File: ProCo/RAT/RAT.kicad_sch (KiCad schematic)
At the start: 40 parts, among them J1 I/O, J2 Power, J3 Power, Q1 2N5458, SW1 SW_SPDT, U1 LM308N

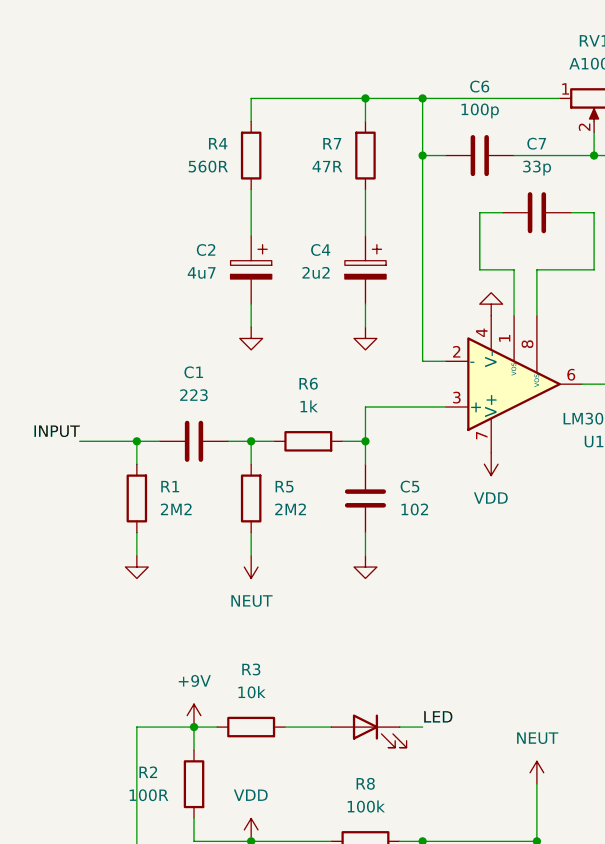
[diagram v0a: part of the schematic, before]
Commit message: refactor: 見直しに伴う形式的な更新
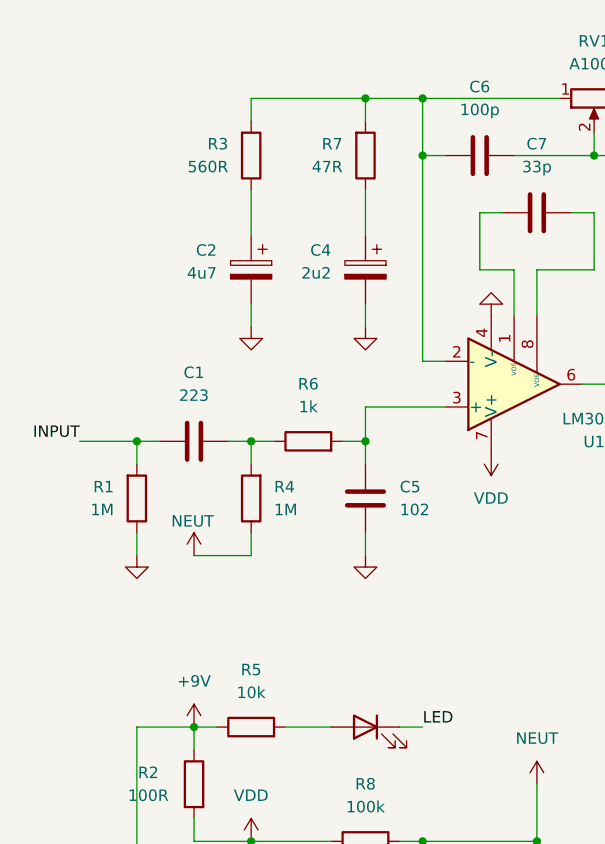
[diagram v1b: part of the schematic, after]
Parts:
- R1: value 2M2 -> 1M
- R4: renamed from R5; value 2M2 -> 1M
- renumbered R4 to R3, R3 to R5
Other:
- moved on the sheet: R1
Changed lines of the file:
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@@
 	(wire
 		(pts
+			(xy 38.1 82.55) (xy 44.45 82.55)
+		)
+		(stroke
+			(width 0)
+			(type default)
+		)
+	)
+	(wire
+		(pts
 			(xy 76.2 107.95) (xy 76.2 114.3)
 		)
@@
 	(wire
 		(pts
+			(xy 44.45 82.55) (xy 44.45 80.01)
+		)
+		(stroke
+			(width 0)
+			(type default)
+		)
+	)
+	(wire
+		(pts
 			(xy 158.75 50.8) (xy 158.75 31.75)
 		)
@@
 	(wire
 		(pts
-			(xy 44.45 80.01) (xy 44.45 82.55)
-		)
-		(stroke
-			(width 0)
-			(type default)
-		)
-	)
-	(wire
-		(pts
 			(xy 44.45 69.85) (xy 44.45 72.39)
 		)
@@
 		(dnp no)
 		(fields_autoplaced yes)
-		(property "Reference" "#PWR025"
+		(property "Reference" "#PWR027"
 			(at 177.8 88.9 0)
 			(hide yes)
@@
 			(project "RAT"
 				(path "/938e6a14-1226-49e6-a6eb-20951bcd3e89"
-					(reference "#PWR025")
+					(reference "#PWR027")
 					(unit 1)
 				)
@@
 		(dnp no)
 		(fields_autoplaced yes)
-		(property "Reference" "#PWR02"
+		(property "Reference" "#PWR03"
 			(at 38.1 105.41 0)
 			(hide yes)
@@
 			(project "RAT"
 				(path "/938e6a14-1226-49e6-a6eb-20951bcd3e89"
-					(reference "#PWR02")
+					(reference "#PWR03")
 					(unit 1)
 				)
@@
 	(symbol
 		(lib_id "Device:R")
-		(at 31.75 76.2 180)
+		(at 31.75 76.2 0)
+		(mirror x)
 		(unit 1)
 		(body_style 1)
@@
 		(in_pos_files yes)
 		(dnp no)
-		(fields_autoplaced yes)
 		(property "Reference" "R1"
-			(at 34.29 74.9299 0)
+			(at 29.21 74.9299 0)
 			(show_name no)
 			(do_not_autoplace no)
@@
 			)
 		)
-		(property "Value" "2M2"
-			(at 34.29 77.4699 0)
+		(property "Value" "1M"
+			(at 29.21 77.4699 0)
 			(show_name no)
 			(do_not_autoplace no)
@@
 		)
 		(property "Footprint" "Resistor_THT:R_Axial_DIN0207_L6.3mm_D2.5mm_P7.62mm_Horizontal"
-			(at 33.528 76.2 90)
+			(at 29.972 76.2 90)
 			(hide yes)
 			(show_name no)
@@
 		(dnp no)
 		(fields_autoplaced yes)
-		(property "Reference" "#PWR023"
+		(property "Reference" "#PWR025"
 			(at 171.45 40.64 0)
 			(hide yes)
@@
 			(project "RAT"
 				(path "/938e6a14-1226-49e6-a6eb-20951bcd3e89"
-					(reference "#PWR023")
+					(reference "#PWR025")
 					(unit 1)
 				)
@@
 		(dnp no)
 		(fields_autoplaced yes)
-		(property "Reference" "R5"
+		(property "Reference" "R4"
 			(at 46.99 74.9299 0)
 			(show_name no)
@@
 			)
 		)
-		(property "Value" "2M2"
+		(property "Value" "1M"
 			(at 46.99 77.4699 0)
 			(show_name no)
@@
 			(project "RAT"
 				(path "/938e6a14-1226-49e6-a6eb-20951bcd3e89"
-					(reference "R5")
+					(reference "R4")
 					(unit 1)
 				)
@@
 	)
 	(symbol
+		(lib_id "power:NEUT")
+		(at 38.1 82.55 0)
+		(unit 1)
+		(body_style 1)
+		(exclude_from_sim no)
+		(in_bom yes)
+		(on_board yes)
+		(in_pos_files yes)
+		(dnp no)
+		(property "Reference" "#PWR05"
+			(at 38.1 86.36 0)
+			(hide yes)
+			(show_name no)
+			(do_not_autoplace no)
+			(effects
+				(font
+					(size 1.27 1.27)
+				)
+			)
+		)
+		(property "Value" "NEUT"
+			(at 35.56 78.74 0)
+			(show_name no)
+			(do_not_autoplace no)
+			(effects
+				(font
+					(size 1.27 1.27)
+				)
+				(justify left)
+			)
+		)
+		(property "Footprint" ""
+			(at 38.1 82.55 0)
+			(hide yes)
+			(show_name no)
+			(do_not_autoplace no)
+			(effects
+				(font
+					(size 1.27 1.27)
+				)
+			)
+		)
+		(property "Datasheet" ""
+			(at 38.1 82.55 0)
+			(hide yes)
+			(show_name no)
+			(do_not_autoplace no)
+			(effects
+				(font
+					(size 1.27 1.27)
+				)
+			)
+		)
+		(property "Description" "Power symbol creates a global label with name \"NEUT\""
+			(at 38.1 82.55 0)
+			(hide yes)
+			(show_name no)
+			(do_not_autoplace no)
+			(effects
+				(font
+					(size 1.27 1.27)
+				)
+			)
+		)
+		(pin "1"
+		)
+		(instances
+			(project "RAT"
+				(path "/938e6a14-1226-49e6-a6eb-20951bcd3e89"
+					(reference "#PWR05")
+					(unit 1)
+				)
+			)
+		)
+	)
+	(symbol
 		(lib_id "power:GND")
 		(at 31.75 127 0)
@@
 		(dnp no)
 		(fields_autoplaced yes)
-		(property "Reference" "#PWR03"
+		(property "Reference" "#PWR02"
 			(at 31.75 133.35 0)
 			(hide yes)
@@
 			(project "RAT"
 				(path "/938e6a14-1226-49e6-a6eb-20951bcd3e89"
-					(reference "#PWR03")
+					(reference "#PWR02")
 					(unit 1)
 				)
@@
 		(dnp no)
 		(fields_autoplaced yes)
-		(property "Reference" "#PWR027"
+		(property "Reference" "#PWR023"
 			(at 171.45 33.02 0)
 			(hide yes)
@@
 			(project "RAT"
 				(path "/938e6a14-1226-49e6-a6eb-20951bcd3e89"
-					(reference "#PWR027")
-					(unit 1)
-				)
-			)
-		)
-	)
-	(symbol
-		(lib_id "power:NEUT")
-		(at 44.45 82.55 180)
-		(unit 1)
-		(body_style 1)
-		(exclude_from_sim no)
-		(in_bom yes)
-		(on_board yes)
-		(in_pos_files yes)
-		(dnp no)
-		(fields_autoplaced yes)
-		(property "Reference" "#PWR05"
-			(at 44.45 78.74 0)
-			(hide yes)
-			(show_name no)
-			(do_not_autoplace no)
-			(effects
-				(font
-					(size 1.27 1.27)
-				)
-			)
-		)
-		(property "Value" "NEUT"
-			(at 44.45 87.63 0)
-			(show_name no)
-			(do_not_autoplace no)
-			(effects
-				(font
-					(size 1.27 1.27)
-				)
-			)
-		)
-		(property "Footprint" ""
-			(at 44.45 82.55 0)
-			(hide yes)
-			(show_name no)
-			(do_not_autoplace no)
-			(effects
-				(font
-					(size 1.27 1.27)
-				)
-			)
-		)
-		(property "Datasheet" ""
-			(at 44.45 82.55 0)
-			(hide yes)
-			(show_name no)
-			(do_not_autoplace no)
-			(effects
-				(font
-					(size 1.27 1.27)
-				)
-			)
-		)
-		(property "Description" "Power symbol creates a global label with name \"NEUT\""
-			(at 44.45 82.55 0)
-			(hide yes)
-			(show_name no)
-			(do_not_autoplace no)
-			(effects
-				(font
-					(size 1.27 1.27)
-				)
-			)
-		)
-		(pin "1"
-		)
-		(instances
-			(project "RAT"
-				(path "/938e6a14-1226-49e6-a6eb-20951bcd3e89"
-					(reference "#PWR05")
+					(reference "#PWR023")
 					(unit 1)
 				)
@@
 		(in_pos_files yes)
 		(dnp no)
-		(property "Reference" "R4"
+		(property "Reference" "R3"
 			(at 41.91 36.8299 0)
 			(show_name no)
@@
 			(project "RAT"
 				(path "/938e6a14-1226-49e6-a6eb-20951bcd3e89"
-					(reference "R4")
+					(reference "R3")
 					(unit 1)
 				)
@@
 		(dnp no)
 		(fields_autoplaced yes)
-		(property "Reference" "R3"
+		(property "Reference" "R5"
 			(at 44.45 95.25 90)
 			(show_name no)
@@
 			(project "RAT"
 				(path "/938e6a14-1226-49e6-a6eb-20951bcd3e89"
-					(reference "R3")
+					(reference "R5")
 					(unit 1)
 				)
